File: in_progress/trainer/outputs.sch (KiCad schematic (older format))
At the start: 38 parts

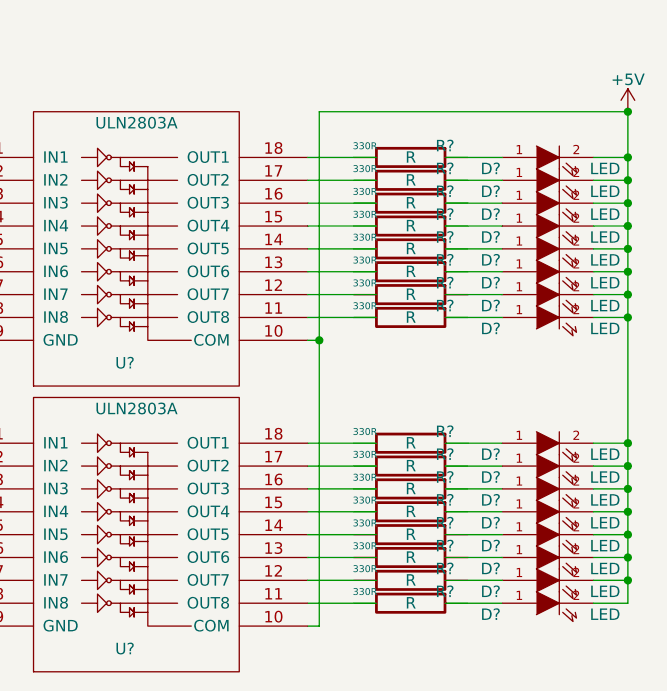
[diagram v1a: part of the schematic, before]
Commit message: .
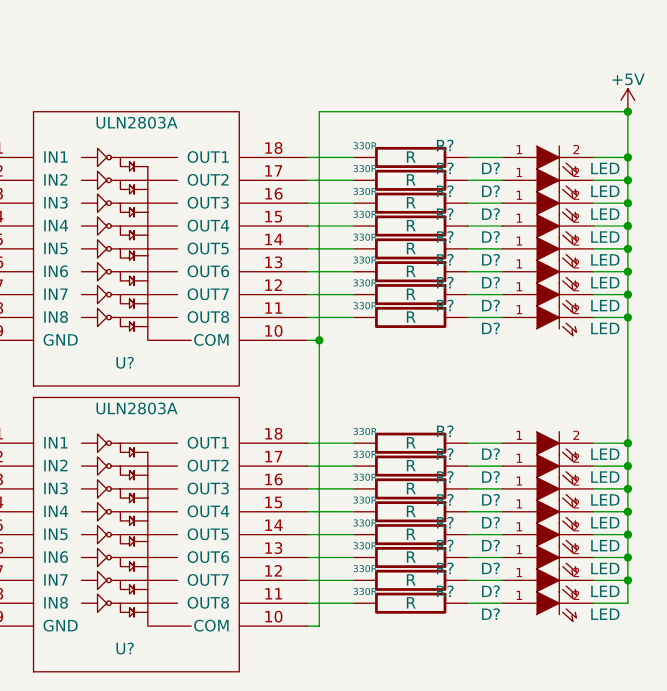
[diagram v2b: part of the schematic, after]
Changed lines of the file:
@@
-EESchema Schematic File Version 2  date 08/12/2015 11:18:57
+EESchema Schematic File Version 2
 LIBS:trainer-rescue
 LIBS:power
@@
 LIBS:valves
 LIBS:MiscellaneousDevices
-LIBS:ULN280xA
 LIBS:Gajda_cmosieee
 LIBS:jhd-162a
 LIBS:capteurs
 LIBS:trainer-cache
-EELAYER 27 0
+EELAYER 25 0
 EELAYER END
 $Descr A4 11693 8268
@@
 	6400 4700 7050 4700
 Wire Wire Line
-	8550 2750 8850 2750
-Wire Wire Line
-	8550 2850 8850 2850
-Wire Wire Line
-	8550 2950 8850 2950
-Wire Wire Line
-	8550 3050 8850 3050
-Wire Wire Line
-	8550 3150 8850 3150
-Wire Wire Line
-	8550 3250 8850 3250
-Wire Wire Line
-	8550 3350 8850 3350
-Wire Wire Line
-	8550 3450 8850 3450
-Wire Wire Line
-	8550 4000 8850 4000
-Wire Wire Line
-	8550 4100 8850 4100
-Wire Wire Line
-	8550 4200 8850 4200
-Wire Wire Line
-	8550 4300 8850 4300
-Wire Wire Line
-	8550 4400 8850 4400
-Wire Wire Line
-	8550 4500 8850 4500
-Wire Wire Line
-	8550 4600 8850 4600
-Wire Wire Line
-	8550 4700 8850 4700
-Wire Wire Line
 	8550 3550 8600 3550
 Wire Wire Line
@@
 Connection ~ 8600 3550
 Wire Wire Line
-	9400 2750 9150 2750
-Wire Wire Line
-	9400 2850 9150 2850
-Wire Wire Line
-	9400 2950 9150 2950
-Wire Wire Line
-	9400 3050 9150 3050
-Wire Wire Line
-	9400 3150 9150 3150
-Wire Wire Line
-	9400 3250 9150 3250
-Wire Wire Line
-	9400 3350 9150 3350
-Wire Wire Line
-	9400 3450 9150 3450
-Wire Wire Line
-	9400 4000 9150 4000
-Wire Wire Line
-	9400 4100 9150 4100
-Wire Wire Line
-	9400 4200 9150 4200
-Wire Wire Line
-	9400 4300 9150 4300
-Wire Wire Line
-	9400 4400 9150 4400
-Wire Wire Line
-	9400 4500 9150 4500
-Wire Wire Line
-	9400 4600 9150 4600
-Wire Wire Line
-	9400 4700 9150 4700
-Wire Wire Line
 	9950 2750 9800 2750
 Wire Wire Line
@@
 Wire Wire Line
 	3000 3850 3000 4600
+Wire Wire Line
+	9250 3450 9400 3450
+Wire Wire Line
+	9250 3350 9400 3350
+Wire Wire Line
+	9250 3250 9400 3250
+Wire Wire Line
+	9250 3150 9400 3150
+Wire Wire Line
+	9250 3050 9400 3050
+Wire Wire Line
+	9250 2950 9400 2950
+Wire Wire Line
+	9250 2850 9400 2850
+Wire Wire Line
+	9250 2750 9400 2750
+Wire Wire Line
+	8550 3350 8750 3350
+Wire Wire Line
+	8550 3250 8750 3250
+Wire Wire Line
+	8550 3150 8750 3150
+Wire Wire Line
+	8550 3050 8750 3050
+Wire Wire Line
+	8550 2950 8750 2950
+Wire Wire Line
+	8550 2850 8750 2850
+Wire Wire Line
+	8550 2750 8750 2750
+Wire Wire Line
+	8750 3450 8550 3450
+Wire Wire Line
+	8550 4000 8750 4000
+Wire Wire Line
+	8550 4100 8750 4100
+Wire Wire Line
+	8550 4200 8750 4200
+Wire Wire Line
+	8550 4300 8750 4300
+Wire Wire Line
+	8550 4400 8750 4400
+Wire Wire Line
+	8550 4500 8750 4500
+Wire Wire Line
+	8550 4600 8750 4600
+Wire Wire Line
+	8550 4700 8750 4700
+Wire Wire Line
+	9250 4000 9400 4000
+Wire Wire Line
+	9250 4100 9400 4100
+Wire Wire Line
+	9400 4200 9250 4200
+Wire Wire Line
+	9250 4300 9400 4300
+Wire Wire Line
+	9400 4400 9250 4400
+Wire Wire Line
+	9250 4500 9400 4500
+Wire Wire Line
+	9400 4600 9250 4600
+Wire Wire Line
+	9250 4700 9400 4700
 $EndSCHEMATC
